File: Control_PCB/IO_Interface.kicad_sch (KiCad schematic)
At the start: 9 parts, among them U6 TCAN1043xDxQ1

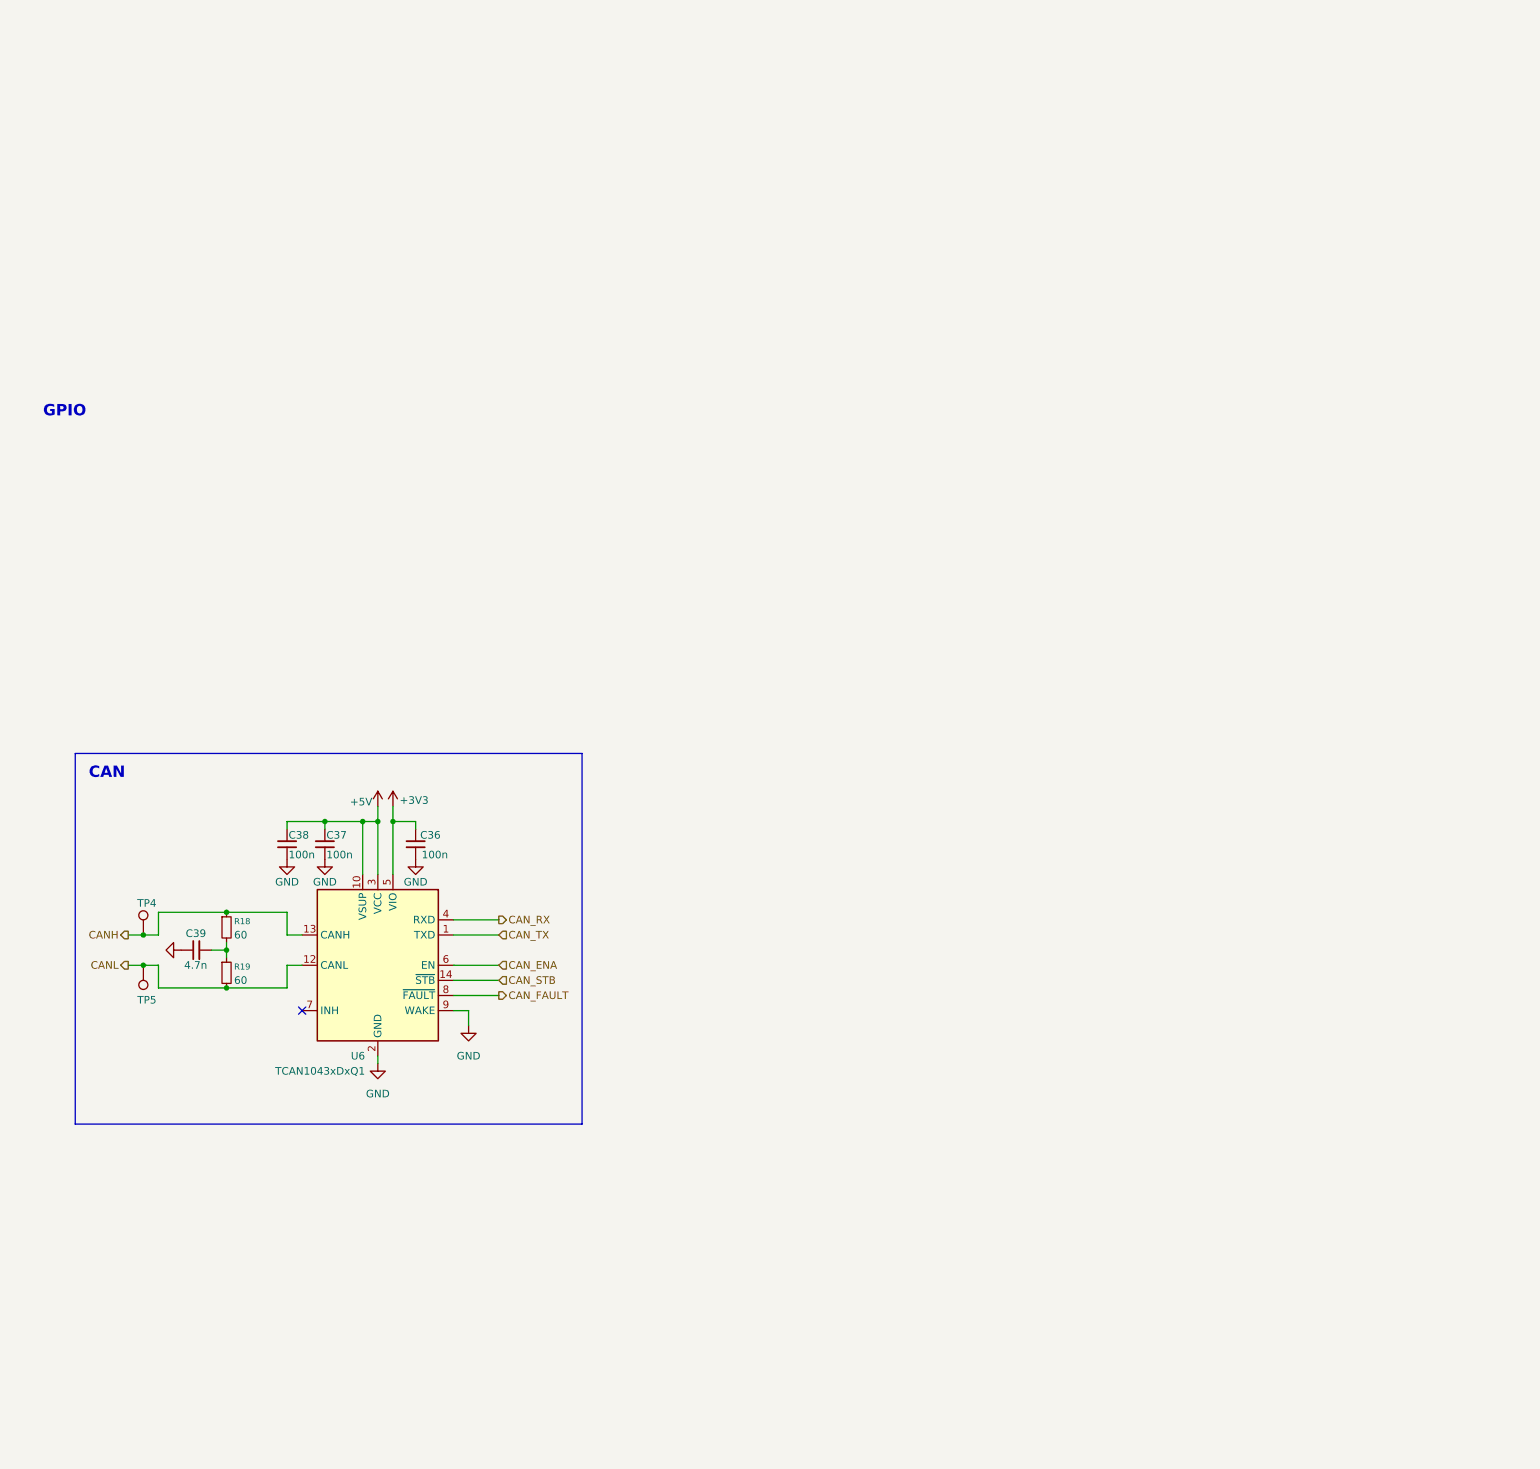
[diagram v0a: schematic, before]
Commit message: 04-10-2026
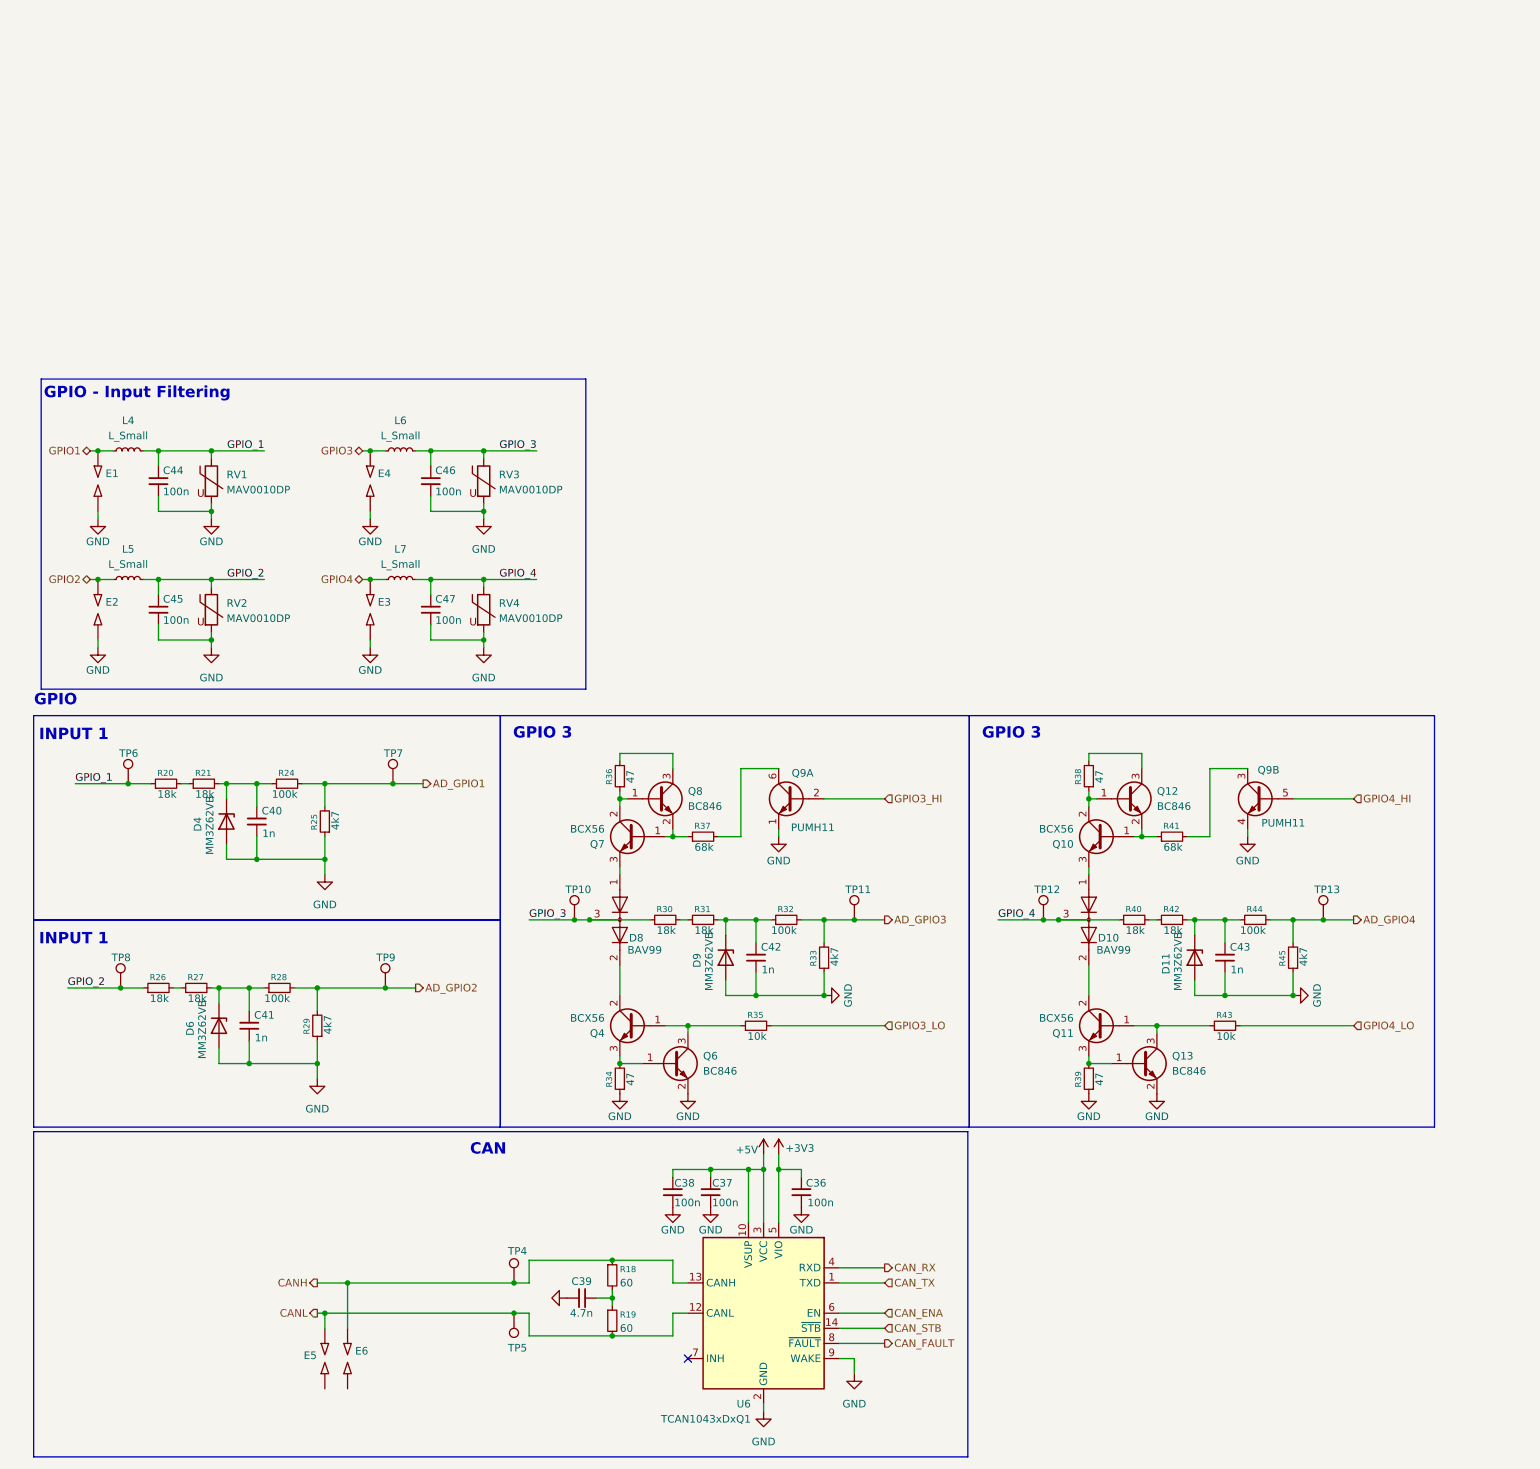
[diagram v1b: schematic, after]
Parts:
- added C40, C41, C42, C43: 1n, Capacitor_SMD:C_0603_1608Metric, symbol Device:C_Small
- added C44, C45, C46, C47: 100n, Package_SO:SOIC-16_3.9x9.9mm_P1.27mm, symbol Device:C_Small
- added D10, D8: BAV99, Package_TO_SOT_SMD:SOT-23, symbol Diode:BAV99
- added D11, D4, D6, D9: MM3Z62VB, Diode_SMD:D_SOD-323F, symbol Diode:MM3Zxx
- added E1, E2, E3, E4, E5, E6: SparkGap, LED_SMD:LED_Kingbright_APFA3010_3x1.5mm_Horizontal, symbol Device:SparkGap
- added L4, L5, L6, L7: L_Small, Package_DFN_QFN:UQFN-20-1EP_3x3mm_P0.4mm_EP1.7x1.7mm_ThermalVias, symbol Device:L_Small
- added Q10, Q11, Q4, Q7: BCX56, Package_TO_SOT_SMD:SOT-89-3, symbol Transistor_BJT:BCX56
- added Q12, Q13, Q6, Q8: BC846, Package_TO_SOT_SMD:SOT-23, symbol Transistor_BJT:BC846
- added Q9: PUMH11, Package_TO_SOT_SMD:SOT-363_SC-70-6, symbol Transistor_BJT:PUMX1
- added R20, R21, R26, R27, R30, R31, R40, R42: 18k, Resistor_SMD:R_0603_1608Metric, symbol Device:R_Small
- added R24, R28, R32, R44: 100k, Resistor_SMD:R_0603_1608Metric, symbol Device:R_Small
- added R25, R29, R33, R45: 4k7, Resistor_SMD:R_0603_1608Metric, symbol Device:R_Small
- added R34, R36, R38, R39: 47, Resistor_SMD:R_0603_1608Metric, symbol Device:R_Small
- added R35, R43: 10k, Resistor_SMD:R_0603_1608Metric, symbol Device:R_Small
- added R37, R41: 68k, Resistor_SMD:R_0603_1608Metric, symbol Device:R_Small
- added RV1, RV2, RV3, RV4: MAV0010DP, symbol Device:Varistor
- added TP10, TP11, TP12, TP13, TP6, TP7, TP8, TP9: TestPoint, TestPoint:TestPoint_Pad_D1.5mm, symbol Connector:TestPoint
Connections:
- net CANH: now also E6.2
- net CANL: now also E5.2
- net GND: now also C40.1, C41.1, C42.1, C43.1, C44.2, C45.2, C46.2, C47.2, D11.2 (A), D4.2 (A), D6.2 (A), D9.2 (A), E1.1, E2.1, E3.1, E4.1, Q13.2 (E), Q6.2 (E), Q9.1 (E1), Q9.4 (E2), R25.1, R29.1, R33.1, R34.1, R39.1, R45.1, RV1.2, RV2.2, RV3.2, RV4.2
- new net: R30.2, R31.1
- new net: C42.2, D9.1 (K), R31.2, R32.1
- new net: Q4.1 (B), Q6.3 (C), R35.1
- new net: D8.2 (A), Q4.2 (C)
- new net: Q4.3 (E), Q6.1 (B), R34.2
- new net: Q7.1 (B), Q8.2 (E), R37.1
- new net: Q7.2 (C), Q8.1 (B), R36.1
- new net: D8.1 (K), Q7.3 (E)
- new net: C43.2, D11.1 (K), R42.2, R44.1
- new net: Q8.3 (C), R36.2
- new net: R20.2, R21.1
- new net: R40.2, R42.1
- new net: Q11.1 (B), Q13.3 (C), R43.1
- new net: D10.2 (A), Q11.2 (C)
- new net: Q11.3 (E), Q13.1 (B), R39.2
- new net: D10.1 (K), Q10.3 (E)
- new net: Q10.2 (C), Q12.1 (B), R38.1
- new net: Q10.1 (B), Q12.2 (E), R41.1
- new net: Q12.3 (C), R38.2
- new net: C40.2, D4.1 (K), R21.2, R24.1
- new net: Q9.6 (C1), R37.2
- new net: C41.2, D6.1 (K), R27.2, R28.1
- new net: R26.2, R27.1
- new net: Q9.3 (C2), R41.2
- new net AD_GPIO1: R24.2, R25.2, TP7.1
- new net AD_GPIO2: R28.2, R29.2, TP9.1
- new net AD_GPIO3: R32.2, R33.2, TP11.1
- new net AD_GPIO4: R44.2, R45.2, TP13.1
- new net GPIO1: E1.2, L4.1
- new net GPIO2: E2.2, L5.1
- new net GPIO3: E4.2, L6.1
- new net GPIO3_HI: Q9.2 (B1)
- new net GPIO3_LO: R35.2
- new net GPIO4: E3.2, L7.1
- new net GPIO4_HI: Q9.5 (B2)
- new net GPIO4_LO: R43.2
- new net GPIO_1: C44.1, L4.2, R20.1, RV1.1, TP6.1
- new net GPIO_2: C45.1, L5.2, R26.1, RV2.1, TP8.1
- new net GPIO_3: C46.1, D8.3 (K), L6.2, R30.1, RV3.1, TP10.1
- new net GPIO_4: C47.1, D10.3 (K), L7.2, R40.1, RV4.1, TP12.1
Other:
- note added: "GPIO - Input Filtering"
- note added: "GPIO 3"
- note added: "INPUT 1"
- moved on the sheet: C36, C37, C38, C39, R18, R19, TP4, TP5, U6

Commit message: 07-20-2026
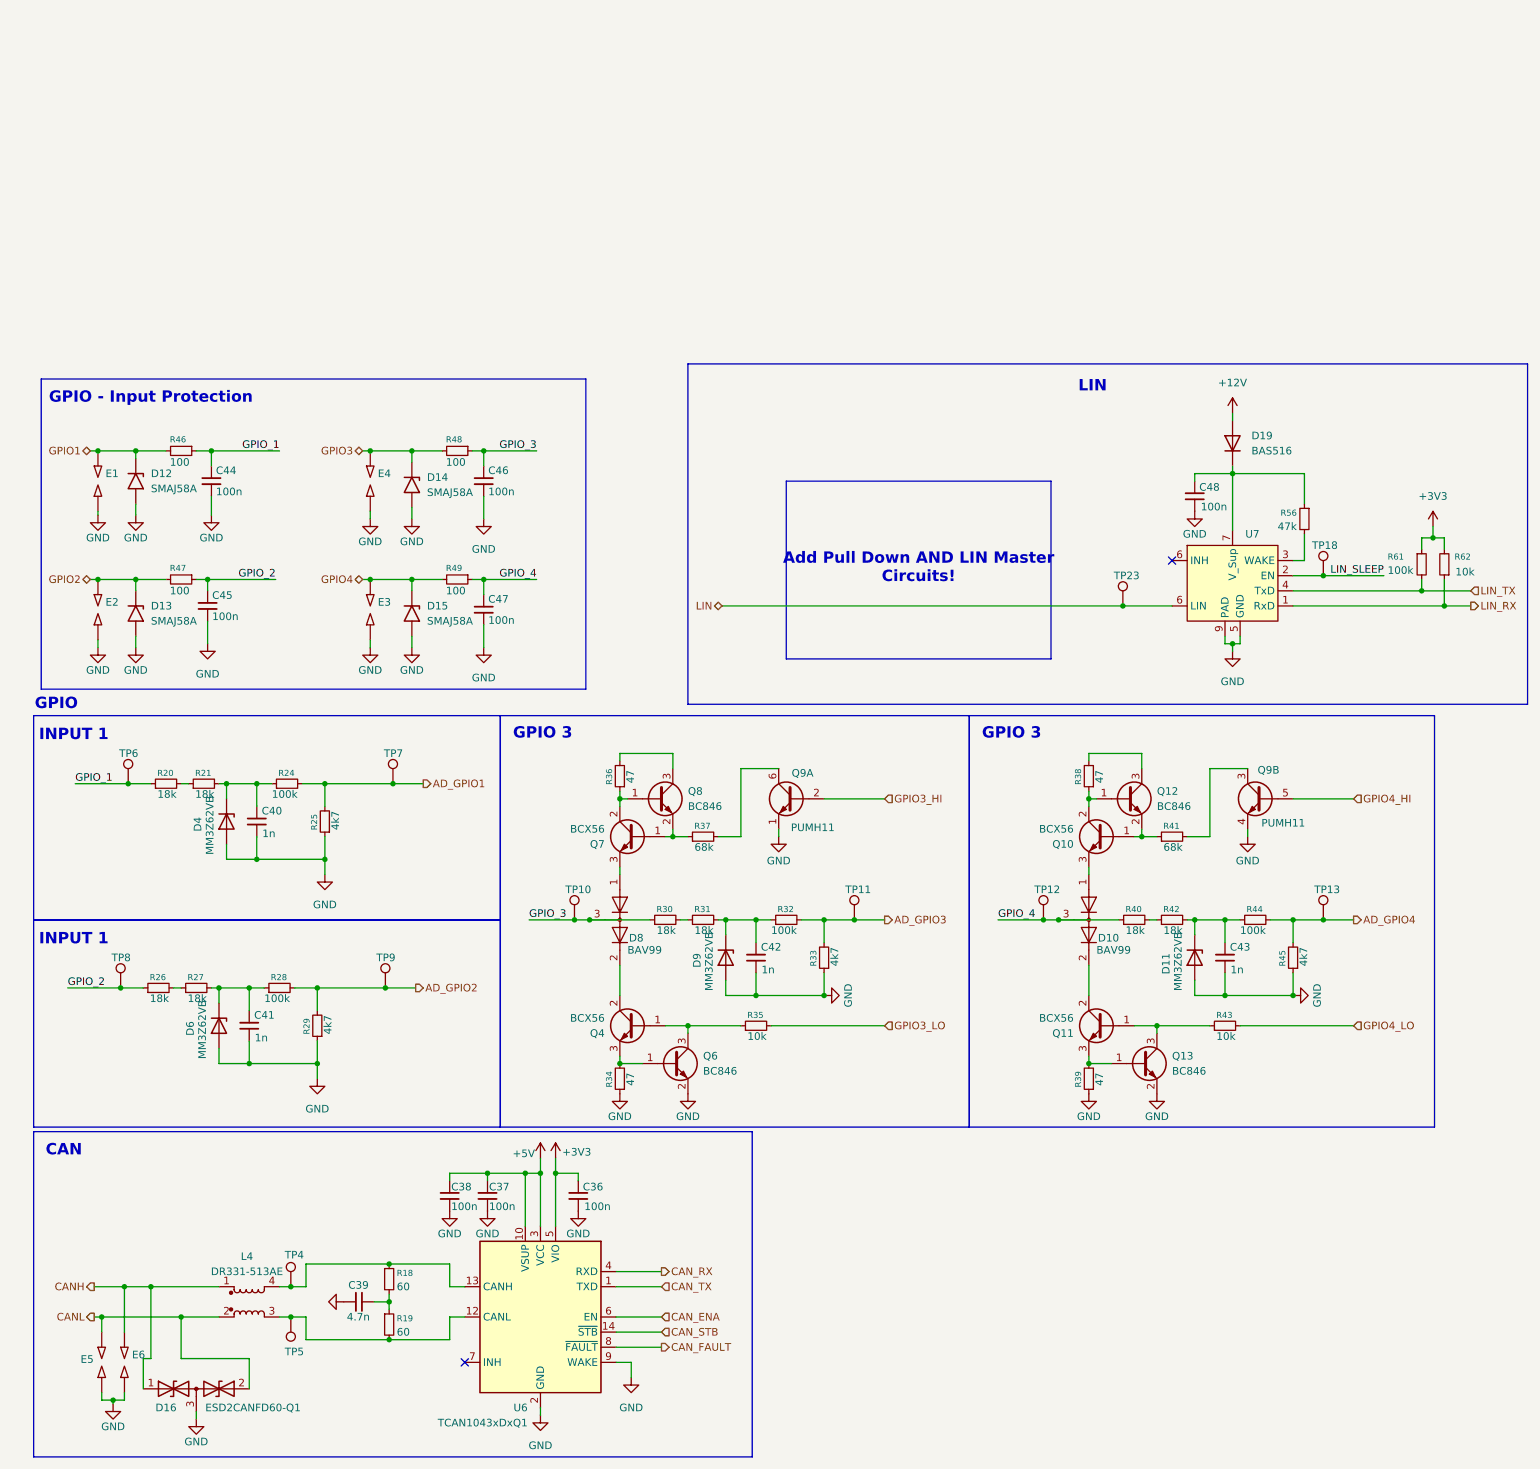
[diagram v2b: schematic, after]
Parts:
- removed L4, L5, L6, L7: L_Small, Package_DFN_QFN:UQFN-20-1EP_3x3mm_P0.4mm_EP1.7x1.7mm_ThermalVias, symbol Device:L_Small
- removed RV1, RV2, RV3, RV4: MAV0010DP, symbol Device:Varistor
- added C48: 100n, Capacitor_SMD:C_0603_1608Metric, symbol Device:C_Small
- added D12, D13, D14, D15: SMAJ58A, Diode_SMD:D_SMA, symbol Diode:SMAJ58A
- added D16: ESD2CANFD60-Q1, Package_TO_SOT_SMD:SOT-23-3, symbol Device:D_TVS_Dual_AAC
- added D19: BAS516, Diode_SMD:D_SOD-523, symbol Diode:BAS516
- added L4: DR331-513AE, Inductor_SMD:L_CommonMode_Bourns_DR331, symbol Device:L_Coupled_1423
- added R46, R47, R48, R49: 100, Resistor_SMD:R_1206_3216Metric, symbol Device:R_Small
- added R56: 47k, symbol Device:R_Small
- added R61: 100k, symbol Device:R_Small
- added R62: 10k, symbol Device:R_Small
- added TP18, TP23: TestPoint, TestPoint:TestPoint_Pad_D1.5mm, symbol Connector:TestPoint
- added U7: (no value), symbol Control_PCB:TLIN2021
- C44, C45, C46, C47: footprint Package_SO:SOIC-16_3.9x9.9mm_P1.27mm -> (none)
- E1, E2, E3, E4, E5, E6: footprint LED_SMD:LED_Kingbright_APFA3010_3x1.5mm_Horizontal -> Control_PCB:Sparkgap_2021-09-02
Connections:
- net +3V3: now also R61.1, R62.2
- net CANH: now also D16.1 (A1), L4.1; no longer R18.1, TP4.1, U6.13 (CANH)
- net CANL: now also D16.2 (A2), L4.2; no longer R19.2, TP5.1, U6.12 (CANL)
- net GND: now also E5.1, E6.1, C48.2, D12.2 (A2), D13.2 (A2), D14.2 (A2), D15.2 (A2), D16.3 (common), U7.5 (GND), U7.9 (PAD)
- net GPIO1: now also D12.1 (A1), R46.2
- net GPIO2: now also D13.1 (A1), R47.2
- net GPIO3: now also D14.1 (A1), R48.2
- net GPIO4: now also D15.1 (A1), R49.2
- net GPIO_1: now also R46.1
- net GPIO_2: now also R47.1
- net GPIO_3: now also R48.1
- net GPIO_4: now also R49.1
- new net: L4.3, R19.2, TP5.1, U6.12 (CANL)
- new net: L4.4, R18.1, TP4.1, U6.13 (CANH)
- new net: C48.1, D19.1 (K), R56.1, U7.7 (V_Sup)
- new net: R56.2, U7.3 (WAKE)
- new net +12V: D19.2 (A)
- new net LIN: TP23.1, U7.6 (LIN)
- new net LIN_RX: R62.1, U7.1 (RxD)
- new net LIN_SLEEP: TP18.1, U7.2 (EN)
- new net LIN_TX: R61.2, U7.4 (TxD)
- no-connect marks 1 -> 2
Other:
- note added: "Add Pull Down AND LIN Master Circuits!"
- note added: "GPIO - Input Protection"
- note added: "LIN"
- note removed: "GPIO - Input Filtering"
- moved on the sheet: C36, C37, C38, C39, C44, C45, C46, C47, E5, E6, R18, R19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

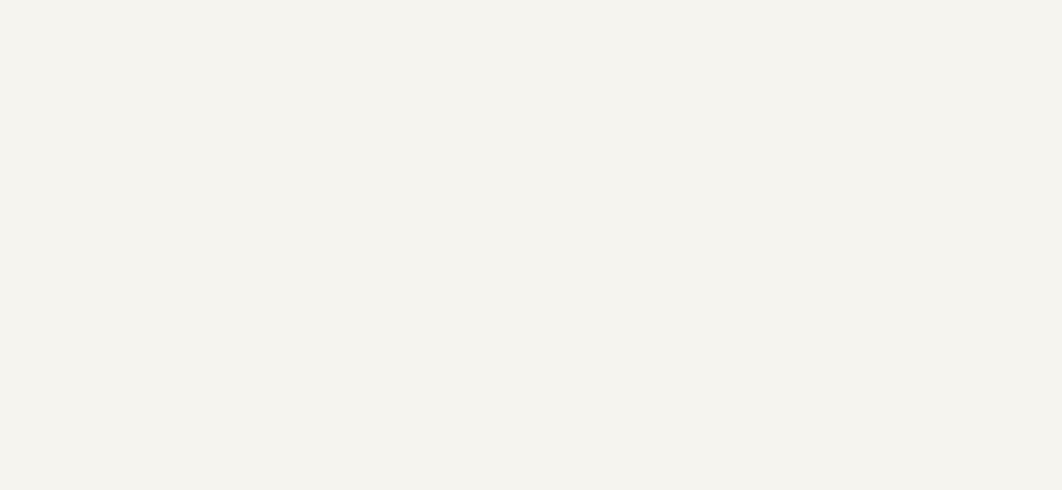
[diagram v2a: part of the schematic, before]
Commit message: 10-10-2026
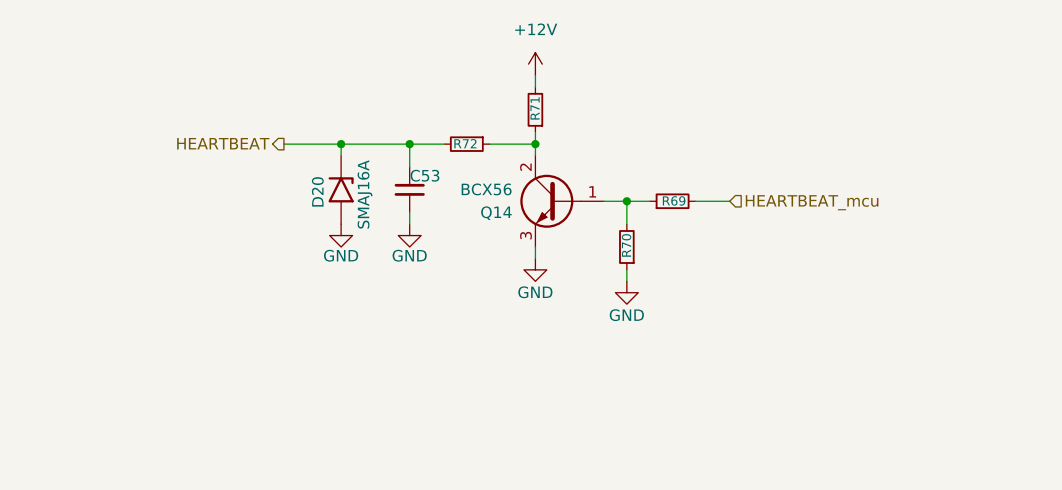
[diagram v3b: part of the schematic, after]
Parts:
- added C53: C_Small, Package_LCC:PLCC-44_16.6x16.6mm_P1.27mm, symbol Device:C_Small
- added D20: SMAJ16A, Diode_SMD:D_SMA, symbol Diode:SMAJ58A
- added Q14: BCX56, Package_TO_SOT_SMD:SOT-89-3, symbol Transistor_BJT:BCX56
- added R69: 1k, Resistor_SMD:R_0603_1608Metric, symbol Device:R_Small
- added R70, R71, R72: 100k, Resistor_SMD:R_0603_1608Metric, symbol Device:R_Small
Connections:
- net +12V: now also R71.2
- net GND: now also C53.2, D20.2 (A2), Q14.3 (E), R70.1
- new net: Q14.1 (B), R69.1, R70.2
- new net: Q14.2 (C), R71.1, R72.1
- new net HEARTBEAT: C53.1, D20.1 (A1), R72.2
- new net HEARTBEAT_mcu: R69.2
